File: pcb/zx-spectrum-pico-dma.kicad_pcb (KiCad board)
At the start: 2 copper layers, 1 part, among them U101 RP2350_Stamp_XL

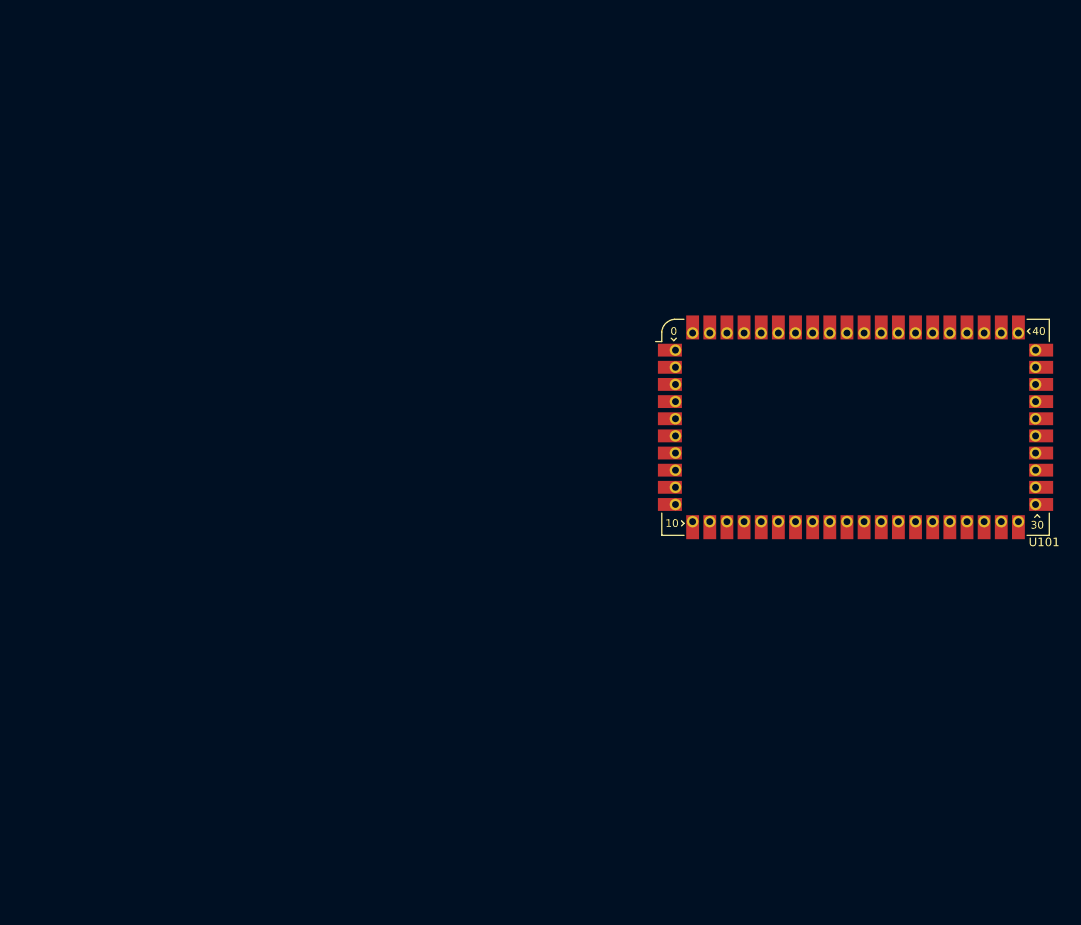
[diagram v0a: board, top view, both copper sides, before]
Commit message: pull in board from zx diagnostics project
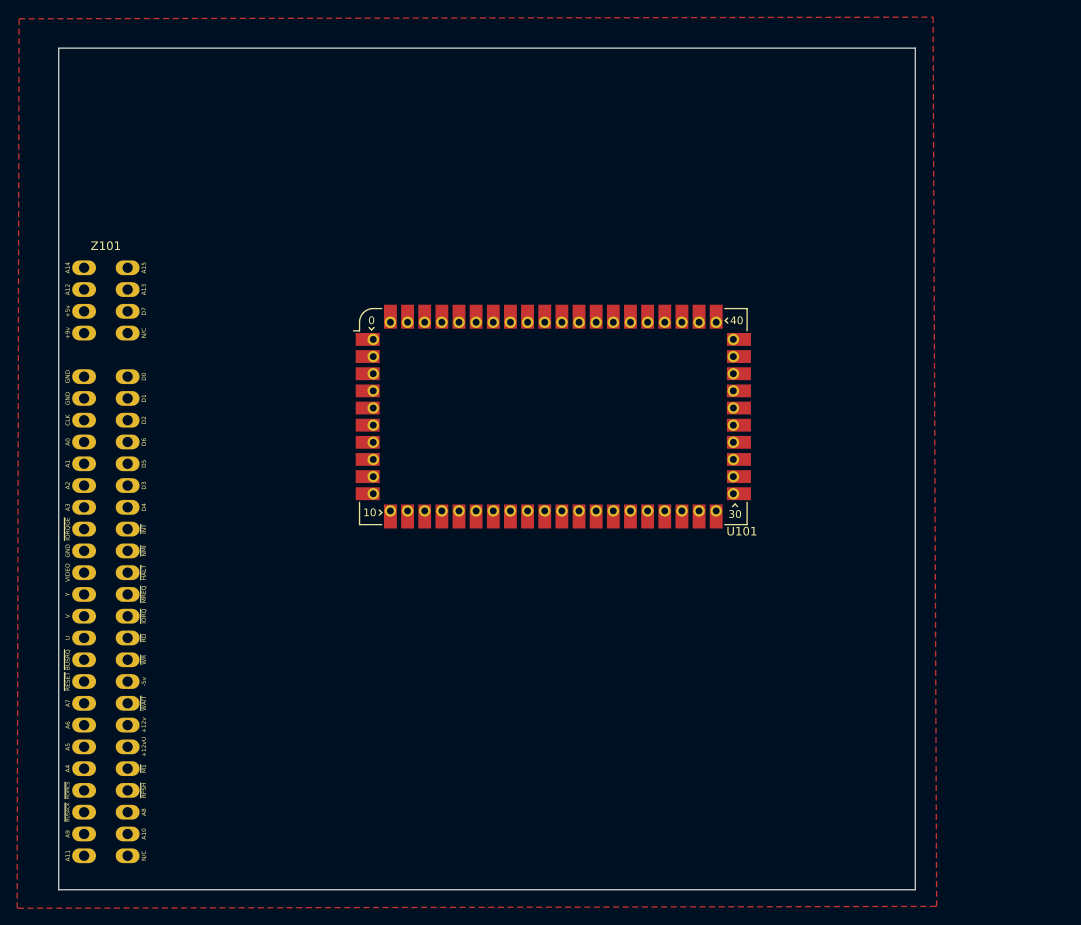
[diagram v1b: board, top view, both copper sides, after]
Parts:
- added Z101: ZX48Bus, zxedge:Spectrum_Edge_Connector, F.Cu at (51.8, 109.5)
- moved U101 35.3 mm to (104.0, 93.8)
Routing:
- added copper zone on F.Cu, net (none)
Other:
- board outline added: 99.9 x 98.2 mm
